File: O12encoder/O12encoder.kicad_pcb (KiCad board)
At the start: 2 copper layers, 14 x 14 mm, 17 parts, among them J1 Conn_01x06_Pin, J2 Conn_01x06_Pin, J3 Conn_01x06_Pin, J4 Conn_01x06_Pin, J5 JST_SM02B-SRSS-TB(LF)(SN), J6 Conn_01x06_Pin, J7 Conn_01x06_Pin, J8 Conn_01x06_Pin, U1 MA702GQ-P, U2 STM32L011F4Ux, U3 THVD1420DRLR

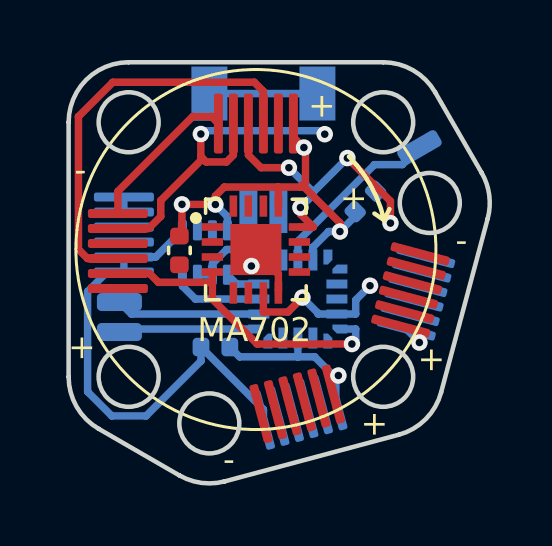
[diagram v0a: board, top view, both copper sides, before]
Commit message: Revert "encoder change to both sides FFC"
This reverts commit 631d04212b57ce457fbe4c2d518c1d39f3519578.
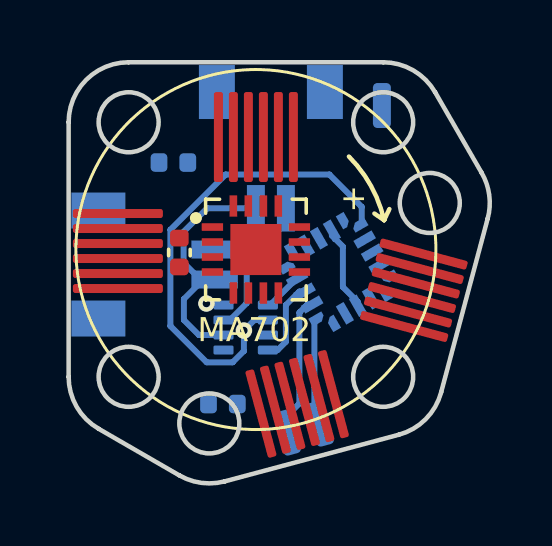
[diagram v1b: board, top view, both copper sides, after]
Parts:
- removed J7, J8: Conn_01x06_Pin, O32controller:FFC_0.5mm_6p
- J5: value JST_SM02B-SRSS-TB(LF)(SN) -> SM02B-SRSS-TB_LF__SN_
- J6: value Conn_01x06_Pin -> SM02B-SRSS-TB_LF__SN_; footprint O32controller:FFC_0.5mm_6p -> O32controller:JST_SM02B-SRSS-TB(LF)(SN)
- U1: value MA702GQ-P -> QFN-3x3_MA702_MNP
- moved TP2 7.36 mm to (52.1, 55.8), turned to -165 degrees
- moved TP3 7.09 mm to (51.0, 56.1), turned to -165 degrees
- moved C3 6.53 mm to (47.2, 47.1), turned to 0 degrees
- moved J6 6.39 mm to (50.5, 46.6)
- moved J5 5.23 mm to (46.6, 50.5), turned to 90 degrees
- moved U3 2.85 mm to (49.7, 52.6), turned to 180 degrees
- moved J4 2.48 mm to (54.9, 52.6), turned to 165 degrees
- moved C2 1.92 mm to (48.9, 55.1)
- moved TP1 1.88 mm to (54.2, 45.2), turned to 180 degrees
- moved U2 1.62 mm to (52.8, 50.8), turned to -60 degrees
- moved J2 0.45 mm to (48.8, 46.2)
- moved C1 0.07 mm to (47.5, 50.1), turned to 90 degrees
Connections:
- net /NRST renamed Net-(U2-NRST)
- J6 pad 1: GND -> /RS485_A
- J6 pad 2: GND -> /RS485_B
- U1 pad 5: /~{MAG2_CS} -> /~{MAG1_CS}
- U2 pad 1: /UART_DE -> unconnected-(U2-PC14-Pad1)
- U2 pad 11: unconnected-(U2-PB1-Pad11) -> /SPI_MOSI
- U2 pad 20: GND -> unconnected-(U2-PB9-Pad20)
- U2 pad 5: /ADC_IN0/WKUP -> unconnected-(U2-PA0-Pad5)
- U2 pad 6: unconnected-(U2-PA1-Pad6) -> /UART_DE
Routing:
- net GND: track 23.9 -> 0.00 mm, vias 1 -> 0
- net /SPI_MISO: track 19.0 -> 0.00 mm, vias 2 -> 0
- net +3.3V: track 20.5 -> 3.45 mm, vias 6 -> 1
- net /UART_DE: track 2.99 -> 16.0 mm, vias 0 -> 1
- net /~{MAG2_CS}: track 11.4 -> 0.00 mm, vias 2 -> 0
- net /SPI_MOSI: track 10.5 -> 0.00 mm, vias 1 -> 0
- net /SPI_SCLK: track 10.1 -> 0.00 mm, vias 4 -> 0
- net /RS485_A: track 0.00 -> 8.44 mm
- net /RS485_B: track 0.00 -> 7.08 mm
- net Net-(U2-NRST): track 5.97 -> 0.00 mm
- net unconnected-(J5-Shield-PadS1): track 3.60 -> 0.00 mm
- net /SWDIO: track 4.52 -> 3.54 mm
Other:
- board text removed: "-"

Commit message: use kicad backup 2am
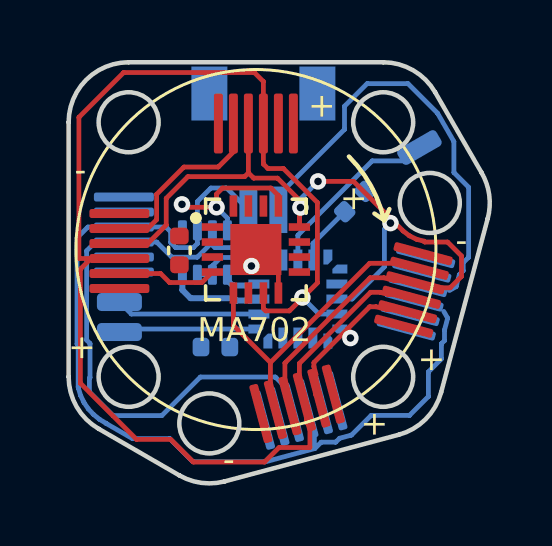
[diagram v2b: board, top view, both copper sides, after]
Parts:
- added J7: Conn_01x06_Pin, O32controller:FFC_0.5mm_6p, B.Cu at (55.7, 50.2)
- added J8: Conn_01x06_Pin, O32controller:FFC_0.5mm_6p, B.Cu at (50.3, 55.7)
- J5: value SM02B-SRSS-TB_LF__SN_ -> JST_SM02B-SRSS-TB(LF)(SN)
- J6: value SM02B-SRSS-TB_LF__SN_ -> Conn_01x06_Pin; footprint O32controller:JST_SM02B-SRSS-TB(LF)(SN) -> O32controller:FFC_0.5mm_6p
- U1: value QFN-3x3_MA702_MNP -> MA702GQ-P
- moved TP2 7.36 mm to (45.5, 52.8), turned to -90 degrees
- moved TP3 7.09 mm to (45.5, 51.8), turned to -90 degrees
- moved J6 6.39 mm to (45.6, 50.8)
- moved C3 6.19 mm to (53.3, 48.4), turned to 45 degrees
- moved J5 5.23 mm to (50.2, 46.7), turned to 0 degrees
- moved U3 2.85 mm to (48.3, 50.1), turned to 90 degrees
- moved J4 2.50 mm to (55.6, 50.1), turned to -15 degrees
- moved C2 1.92 mm to (48.6, 53.2)
- moved TP1 1.88 mm to (55.5, 46.6), turned to -60 degrees
- moved U2 1.62 mm to (51.4, 51.6), turned to -90 degrees
- moved J2 0.45 mm to (48.8, 45.8)
- moved C1 0.07 mm to (47.5, 50.0), turned to -90 degrees
- moved J1 0.05 mm to (45.5, 48.8)
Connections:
- net Net-(U2-NRST) renamed /NRST
- J6 pad 1: /RS485_A -> GND
- J6 pad 2: /RS485_B -> GND
- U1 pad 5: /~{MAG1_CS} -> /~{MAG2_CS}
- U2 pad 1: unconnected-(U2-PC14-Pad1) -> /UART_DE
- U2 pad 20: unconnected-(U2-PB9-Pad20) -> GND
- U2 pad 5: unconnected-(U2-PA0-Pad5) -> /ADC_IN0/WKUP
- U2 pad 6: /UART_DE -> unconnected-(U2-PA1-Pad6)
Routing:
- net /SPI_MISO: track 0.00 -> 46.0 mm, vias 0 -> 1
- net /SPI_SCLK: track 0.00 -> 29.2 mm, vias 0 -> 3
- net /RS485_B: track 7.08 -> 35.6 mm
- net /RS485_A: track 8.44 -> 30.8 mm
- net /~{MAG2_CS}: track 0.00 -> 15.3 mm
- net /UART_DE: track 16.0 -> 2.91 mm, vias 1 -> 0
- net /SPI_MOSI: track 0.00 -> 9.29 mm, vias 0 -> 1
- net /NRST: track 0.00 -> 6.04 mm
- net +3.3V: track 3.45 -> 7.15 mm, vias 1 -> 2
- net GND: track 0.00 -> 2.00 mm, vias 0 -> 1
- net /SWDIO: track 3.54 -> 4.52 mm
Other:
- board text added: "-"

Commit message: undo autoroute
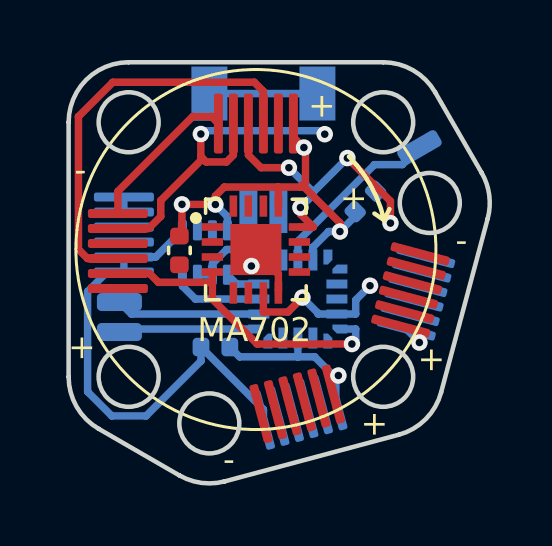
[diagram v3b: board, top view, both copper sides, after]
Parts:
- moved C3 0.35 mm to (53.6, 48.4)
- moved J4 0.10 mm to (55.5, 50.1)
- moved J1 0.05 mm to (45.4, 48.8)
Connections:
- U2 pad 11: /SPI_MOSI -> unconnected-(U2-PB1-Pad11)
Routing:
- net /RS485_B: track 35.6 -> 0.00 mm
- net /RS485_A: track 30.8 -> 0.00 mm
- net /SPI_MISO: track 46.0 -> 19.0 mm, vias 1 -> 2
- net GND: track 2.00 -> 23.9 mm
- net /SPI_SCLK: track 29.2 -> 10.1 mm, vias 3 -> 4
- net +3.3V: track 7.15 -> 20.5 mm, vias 2 -> 6
- net /~{MAG2_CS}: track 15.3 -> 11.4 mm, vias 0 -> 2
- net unconnected-(J5-Shield-PadS1): track 0.00 -> 3.60 mm
- net /SPI_MOSI: track 9.29 -> 10.5 mm
